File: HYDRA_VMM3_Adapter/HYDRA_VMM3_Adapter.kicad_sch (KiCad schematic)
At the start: 6 parts, among them J1 ME1014010101011, J2 ME1014010101011, J3 ME1014010101011, J4 ME1014010101011, J5 ME1014010101011, J6 ME1014010101011

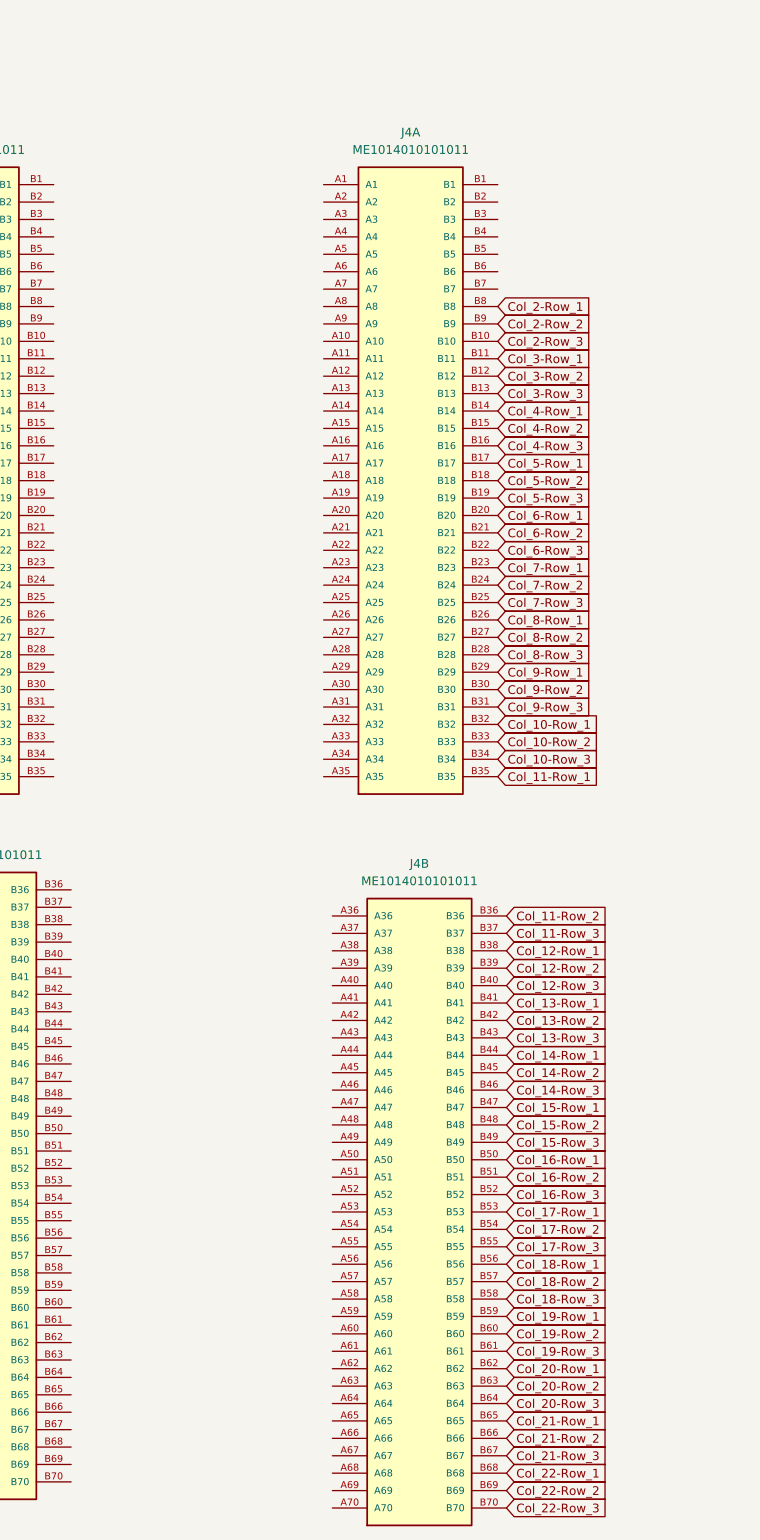
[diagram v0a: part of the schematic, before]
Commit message: .
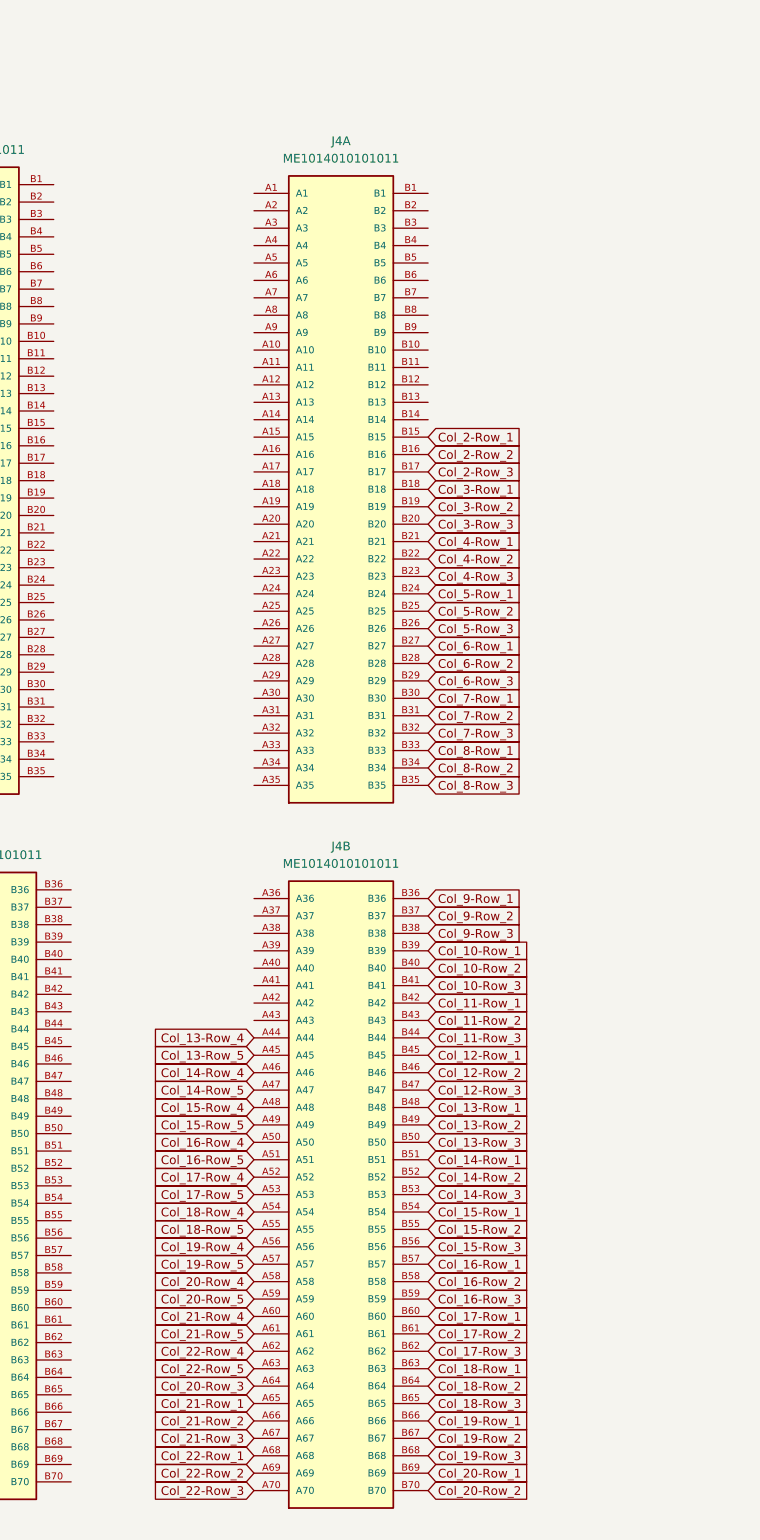
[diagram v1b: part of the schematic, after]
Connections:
- net Col_10-Row_1: now also J4.B39; no longer J4.B32
- net Col_10-Row_2: now also J4.B40; no longer J4.B33
- net Col_10-Row_3: now also J4.B41; no longer J4.B34
- net Col_11-Row_1: now also J4.B42; no longer J4.B35
- net Col_11-Row_2: now also J4.B43; no longer J4.B36
- net Col_11-Row_3: now also J4.B44; no longer J4.B37
- net Col_12-Row_1: now also J4.B45; no longer J4.B38
- net Col_12-Row_2: now also J4.B46; no longer J4.B39
- net Col_12-Row_3: now also J4.B47; no longer J4.B40
- net Col_13-Row_1: now also J4.B48; no longer J4.B41
- net Col_13-Row_2: now also J4.B49; no longer J4.B42
- net Col_13-Row_3: now also J4.B50; no longer J4.B43
- net Col_14-Row_1: now also J4.B51; no longer J4.B44
- net Col_14-Row_2: now also J4.B52; no longer J4.B45
- net Col_14-Row_3: now also J4.B53; no longer J4.B46
- net Col_15-Row_1: now also J4.B54; no longer J4.B47
- net Col_15-Row_2: now also J4.B55; no longer J4.B48
- net Col_15-Row_3: now also J4.B56; no longer J4.B49
- net Col_16-Row_1: now also J4.B57; no longer J4.B50
- net Col_16-Row_2: now also J4.B58; no longer J4.B51
- net Col_16-Row_3: now also J4.B59; no longer J4.B52
- net Col_17-Row_1: now also J4.B60; no longer J4.B53
- net Col_17-Row_2: now also J4.B61; no longer J4.B54
- net Col_17-Row_3: now also J4.B62; no longer J4.B55
- net Col_18-Row_1: now also J4.B63; no longer J4.B56
- net Col_18-Row_2: now also J4.B64; no longer J4.B57
- net Col_18-Row_3: now also J4.B65; no longer J4.B58
- net Col_19-Row_1: now also J4.B66; no longer J4.B59
- net Col_19-Row_2: now also J4.B67; no longer J4.B60
- net Col_19-Row_3: now also J4.B68; no longer J4.B61
- net Col_2-Row_1: now also J4.B15; no longer J4.B8
- net Col_2-Row_2: now also J4.B16; no longer J4.B9
- net Col_2-Row_3: now also J4.B17; no longer J4.B10
- net Col_20-Row_1: now also J4.B69; no longer J4.B62
- net Col_20-Row_2: now also J4.B70; no longer J4.B63
- net Col_20-Row_3: now also J4.A64; no longer J4.B64
- net Col_21-Row_1: now also J4.A65; no longer J4.B65
- net Col_21-Row_2: now also J4.A66; no longer J4.B66
- net Col_21-Row_3: now also J4.A67; no longer J4.B67
- net Col_22-Row_1: now also J4.A68; no longer J4.B68
- net Col_22-Row_2: now also J4.A69; no longer J4.B69
- net Col_22-Row_3: now also J4.A70; no longer J4.B70
- net Col_3-Row_1: now also J4.B18; no longer J4.B11
- net Col_3-Row_2: now also J4.B19; no longer J4.B12
- net Col_3-Row_3: now also J4.B20; no longer J4.B13
- net Col_4-Row_1: now also J4.B21; no longer J4.B14
- net Col_4-Row_2: now also J4.B22; no longer J4.B15
- net Col_4-Row_3: now also J4.B23; no longer J4.B16
- net Col_5-Row_1: now also J4.B24; no longer J4.B17
- net Col_5-Row_2: now also J4.B25; no longer J4.B18
- net Col_5-Row_3: now also J4.B26; no longer J4.B19
- net Col_6-Row_1: now also J4.B27; no longer J4.B20
- net Col_6-Row_2: now also J4.B28; no longer J4.B21
- net Col_6-Row_3: now also J4.B29; no longer J4.B22
- net Col_7-Row_1: now also J4.B30; no longer J4.B23
- net Col_7-Row_2: now also J4.B31; no longer J4.B24
- net Col_7-Row_3: now also J4.B32; no longer J4.B25
- net Col_8-Row_1: now also J4.B33; no longer J4.B26
- net Col_8-Row_2: now also J4.B34; no longer J4.B27
- net Col_8-Row_3: now also J4.B35; no longer J4.B28
- net Col_9-Row_1: now also J4.B36; no longer J4.B29
- net Col_9-Row_2: now also J4.B37; no longer J4.B30
- net Col_9-Row_3: now also J4.B38; no longer J4.B31
- net Col_13-Row_4: now reaches J4.A44
- net Col_13-Row_5: now reaches J4.A45
- net Col_14-Row_4: now reaches J4.A46
- net Col_14-Row_5: now reaches J4.A47
- net Col_15-Row_4: now reaches J4.A48
- net Col_15-Row_5: now reaches J4.A49
- net Col_16-Row_4: now reaches J4.A50
- net Col_16-Row_5: now reaches J4.A51
- net Col_17-Row_4: now reaches J4.A52
- net Col_17-Row_5: now reaches J4.A53
- net Col_18-Row_4: now reaches J4.A54
- net Col_18-Row_5: now reaches J4.A55
- net Col_19-Row_4: now reaches J4.A56
- net Col_19-Row_5: now reaches J4.A57
- net Col_20-Row_4: now reaches J4.A58
- net Col_20-Row_5: now reaches J4.A59
- net Col_21-Row_4: now reaches J4.A60
- net Col_21-Row_5: now reaches J4.A61
- net Col_22-Row_4: now reaches J4.A62
- net Col_22-Row_5: now reaches J4.A63
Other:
- moved on the sheet: J4A, J4B

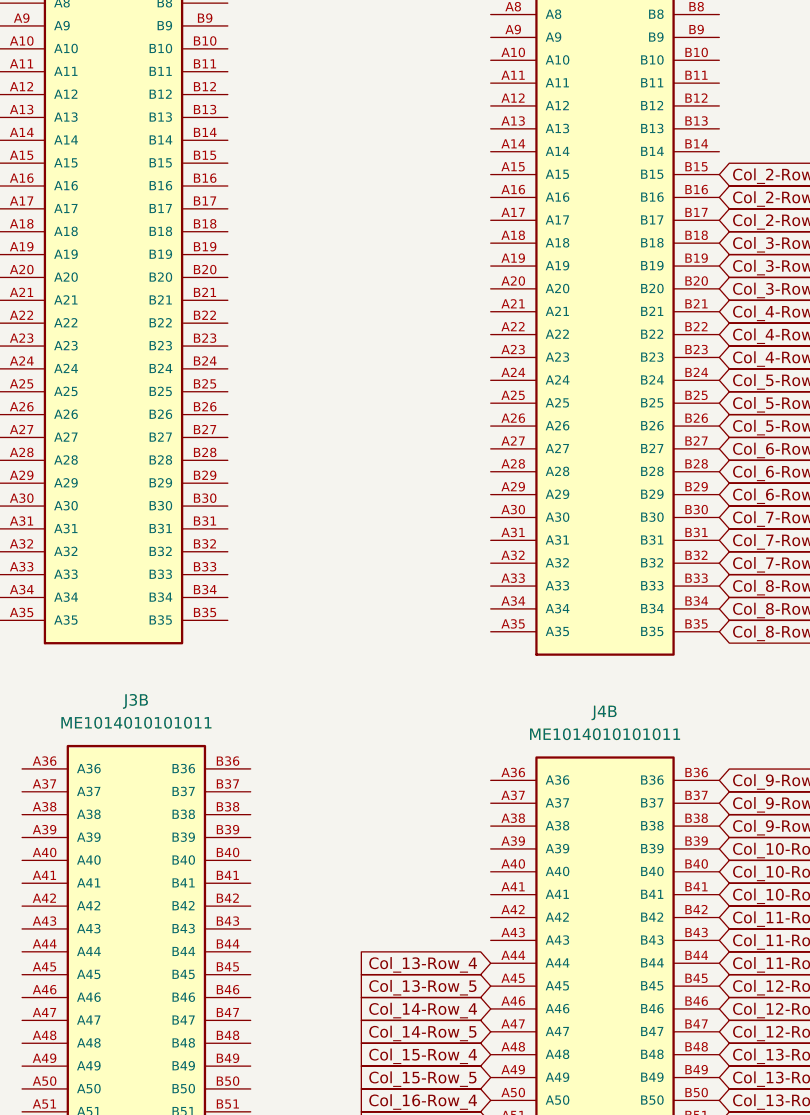
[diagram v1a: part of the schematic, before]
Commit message: .
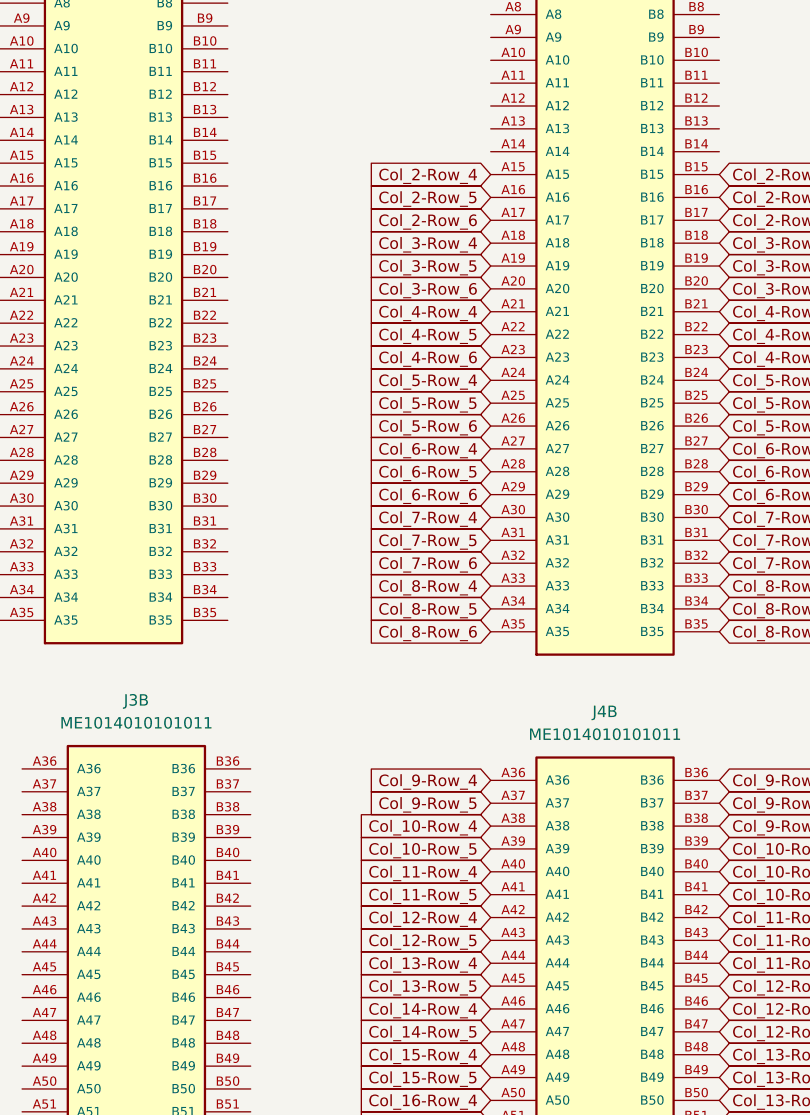
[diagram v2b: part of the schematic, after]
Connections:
- net Col_2-Row_4: now reaches J4.A15
- net Col_2-Row_5: now reaches J4.A16
- net Col_2-Row_6: now reaches J4.A17
- net Col_3-Row_4: now reaches J4.A18
- net Col_3-Row_5: now reaches J4.A19
- net Col_3-Row_6: now reaches J4.A20
- net Col_4-Row_4: now reaches J4.A21
- net Col_4-Row_5: now reaches J4.A22
- net Col_4-Row_6: now reaches J4.A23
- net Col_5-Row_4: now reaches J4.A24
- net Col_5-Row_5: now reaches J4.A25
- net Col_5-Row_6: now reaches J4.A26
- net Col_6-Row_4: now reaches J4.A27
- net Col_6-Row_5: now reaches J4.A28
- net Col_6-Row_6: now reaches J4.A29
- net Col_7-Row_4: now reaches J4.A30
- net Col_7-Row_5: now reaches J4.A31
- net Col_7-Row_6: now reaches J4.A32
- net Col_8-Row_4: now reaches J4.A33
- net Col_8-Row_5: now reaches J4.A34
- net Col_8-Row_6: now reaches J4.A35
- net Col_9-Row_4: now reaches J4.A36
- net Col_9-Row_5: now reaches J4.A37
- net Col_10-Row_4: now reaches J4.A38
- net Col_10-Row_5: now reaches J4.A39
- net Col_11-Row_4: now reaches J4.A40
- net Col_11-Row_5: now reaches J4.A41
- net Col_12-Row_4: now reaches J4.A42
- net Col_12-Row_5: now reaches J4.A43

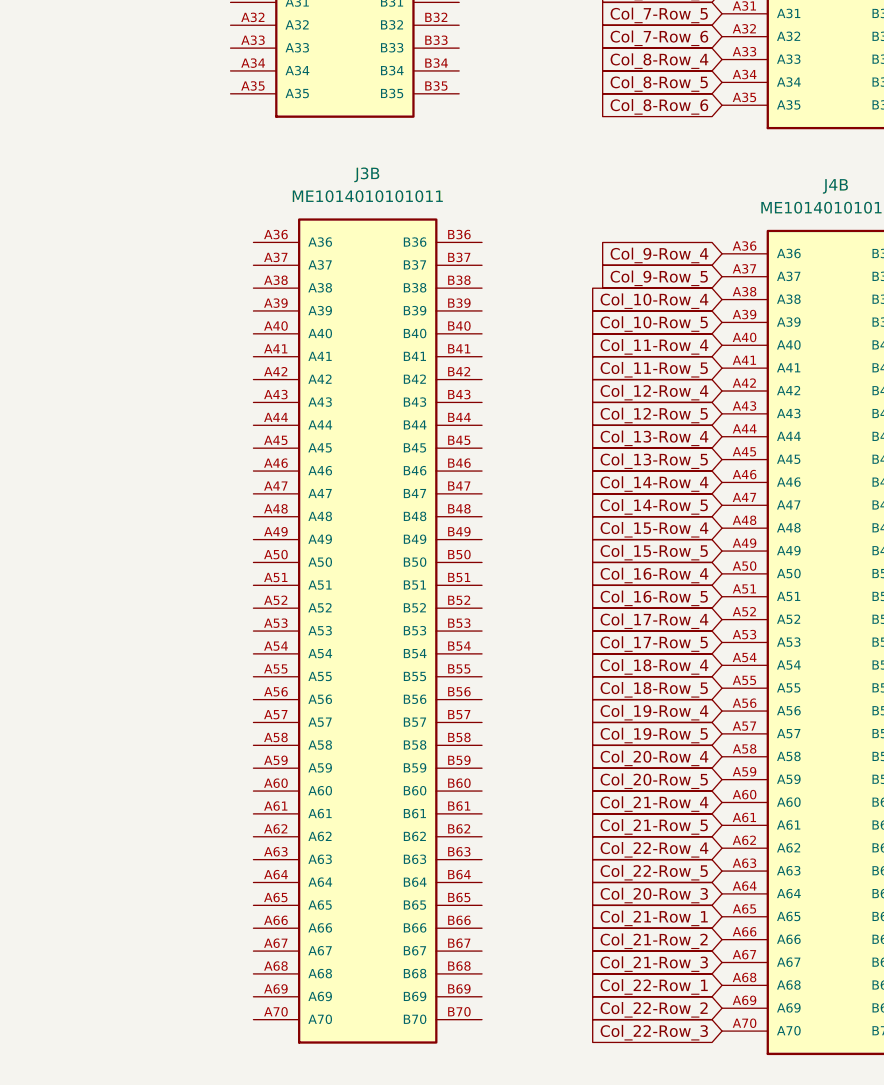
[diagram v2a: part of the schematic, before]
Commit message: .
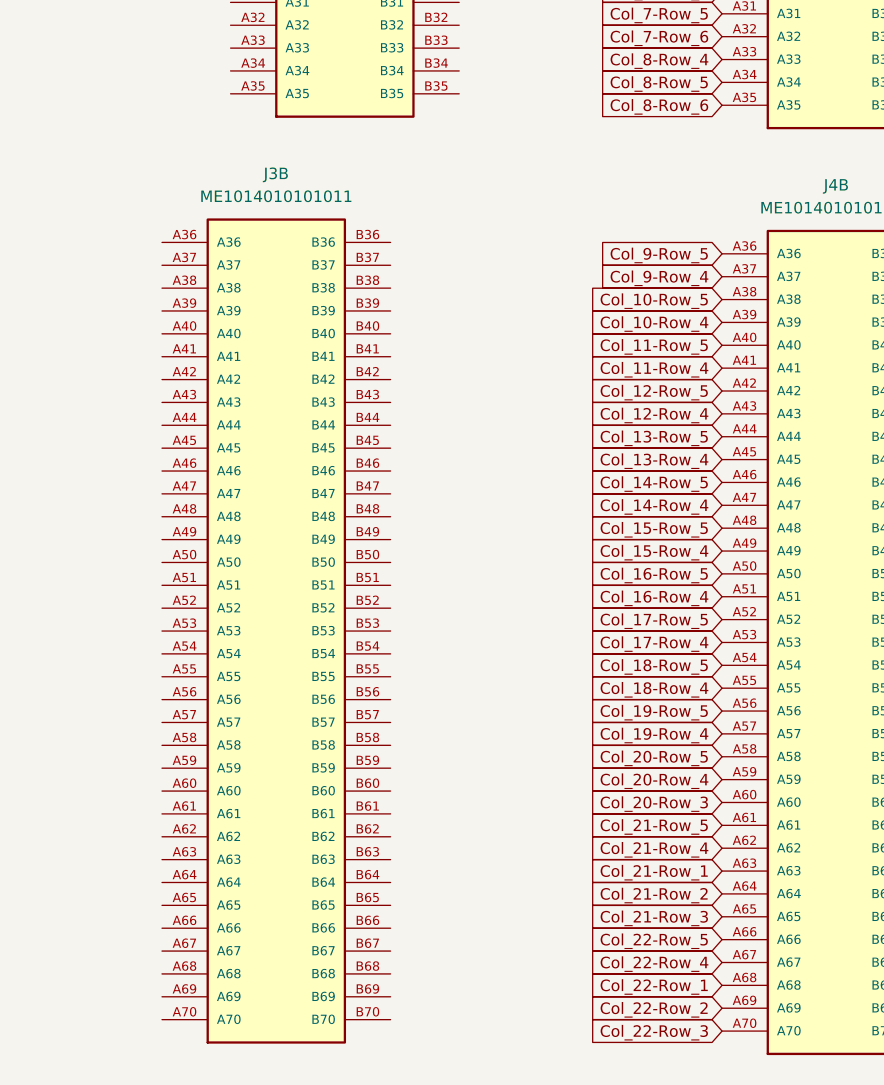
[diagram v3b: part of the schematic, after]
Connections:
- net Col_10-Row_4: now also J4.A39; no longer J4.A38
- net Col_10-Row_5: now also J4.A38; no longer J4.A39
- net Col_11-Row_4: now also J4.A41; no longer J4.A40
- net Col_11-Row_5: now also J4.A40; no longer J4.A41
- net Col_12-Row_4: now also J4.A43; no longer J4.A42
- net Col_12-Row_5: now also J4.A42; no longer J4.A43
- net Col_13-Row_4: now also J4.A45; no longer J4.A44
- net Col_13-Row_5: now also J4.A44; no longer J4.A45
- net Col_14-Row_4: now also J4.A47; no longer J4.A46
- net Col_14-Row_5: now also J4.A46; no longer J4.A47
- net Col_15-Row_4: now also J4.A49; no longer J4.A48
- net Col_15-Row_5: now also J4.A48; no longer J4.A49
- net Col_16-Row_4: now also J4.A51; no longer J4.A50
- net Col_16-Row_5: now also J4.A50; no longer J4.A51
- net Col_17-Row_4: now also J4.A53; no longer J4.A52
- net Col_17-Row_5: now also J4.A52; no longer J4.A53
- net Col_18-Row_4: now also J4.A55; no longer J4.A54
- net Col_18-Row_5: now also J4.A54; no longer J4.A55
- net Col_19-Row_4: now also J4.A57; no longer J4.A56
- net Col_19-Row_5: now also J4.A56; no longer J4.A57
- net Col_20-Row_3: now also J4.A60; no longer J4.A64
- net Col_20-Row_4: now also J4.A59; no longer J4.A58
- net Col_20-Row_5: now also J4.A58; no longer J4.A59
- net Col_21-Row_1: now also J4.A63; no longer J4.A65
- net Col_21-Row_2: now also J4.A64; no longer J4.A66
- net Col_21-Row_3: now also J4.A65; no longer J4.A67
- net Col_21-Row_4: now also J4.A62; no longer J4.A60
- net Col_22-Row_4: now also J4.A67; no longer J4.A62
- net Col_22-Row_5: now also J4.A66; no longer J4.A63
- net Col_9-Row_4: now also J4.A37; no longer J4.A36
- net Col_9-Row_5: now also J4.A36; no longer J4.A37
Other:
- moved on the sheet: J3B
